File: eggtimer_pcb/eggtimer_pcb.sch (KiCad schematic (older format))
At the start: 84 parts, among them J1 Conn_01x03, Q1 CPH3350-TL-W, Q10 2N7002P,215, Q2 CPH3350-TL-W, Q3 CPH3350-TL-W, Q4 CPH3350-TL-W, Q5 CPH3350-TL-W, Q6 CPH3350-TL-W, Q7 CPH3350-TL-W, Q8 CPH3350-TL-W, Q9 2N7002P,215, SW1 Rotary_Encoder_Switch, SW2 SW_Push, U1 BD70522GUL-E2, U2 STM32G051GxU, Y1 32.xxxk

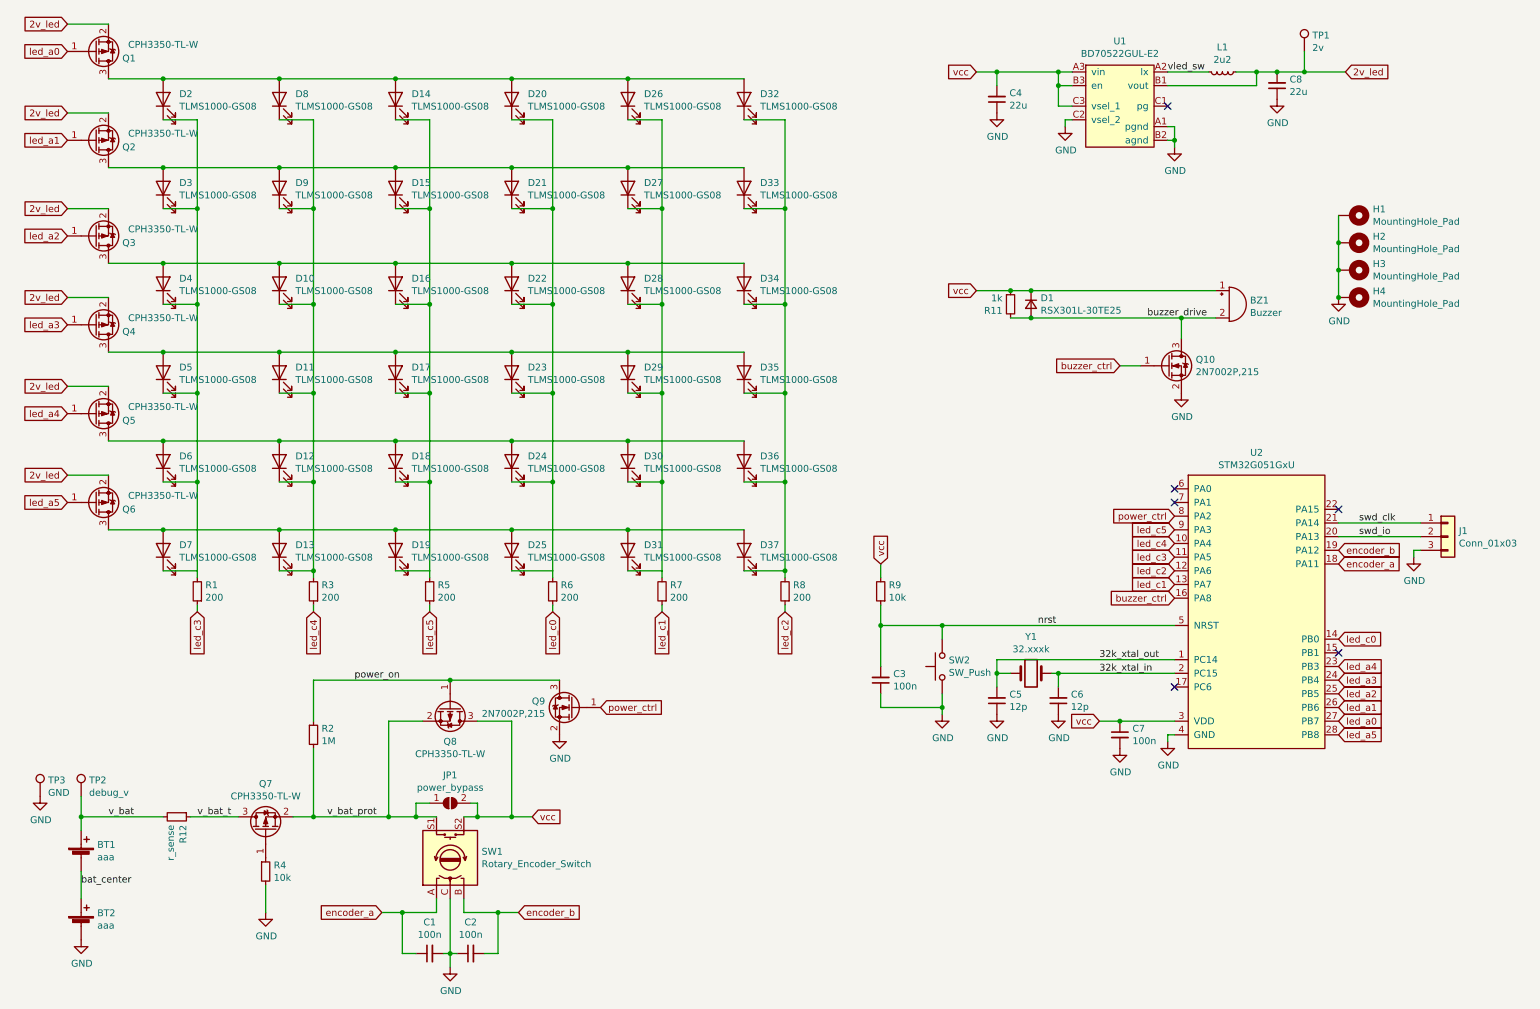
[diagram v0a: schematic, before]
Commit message: MORE LEDS
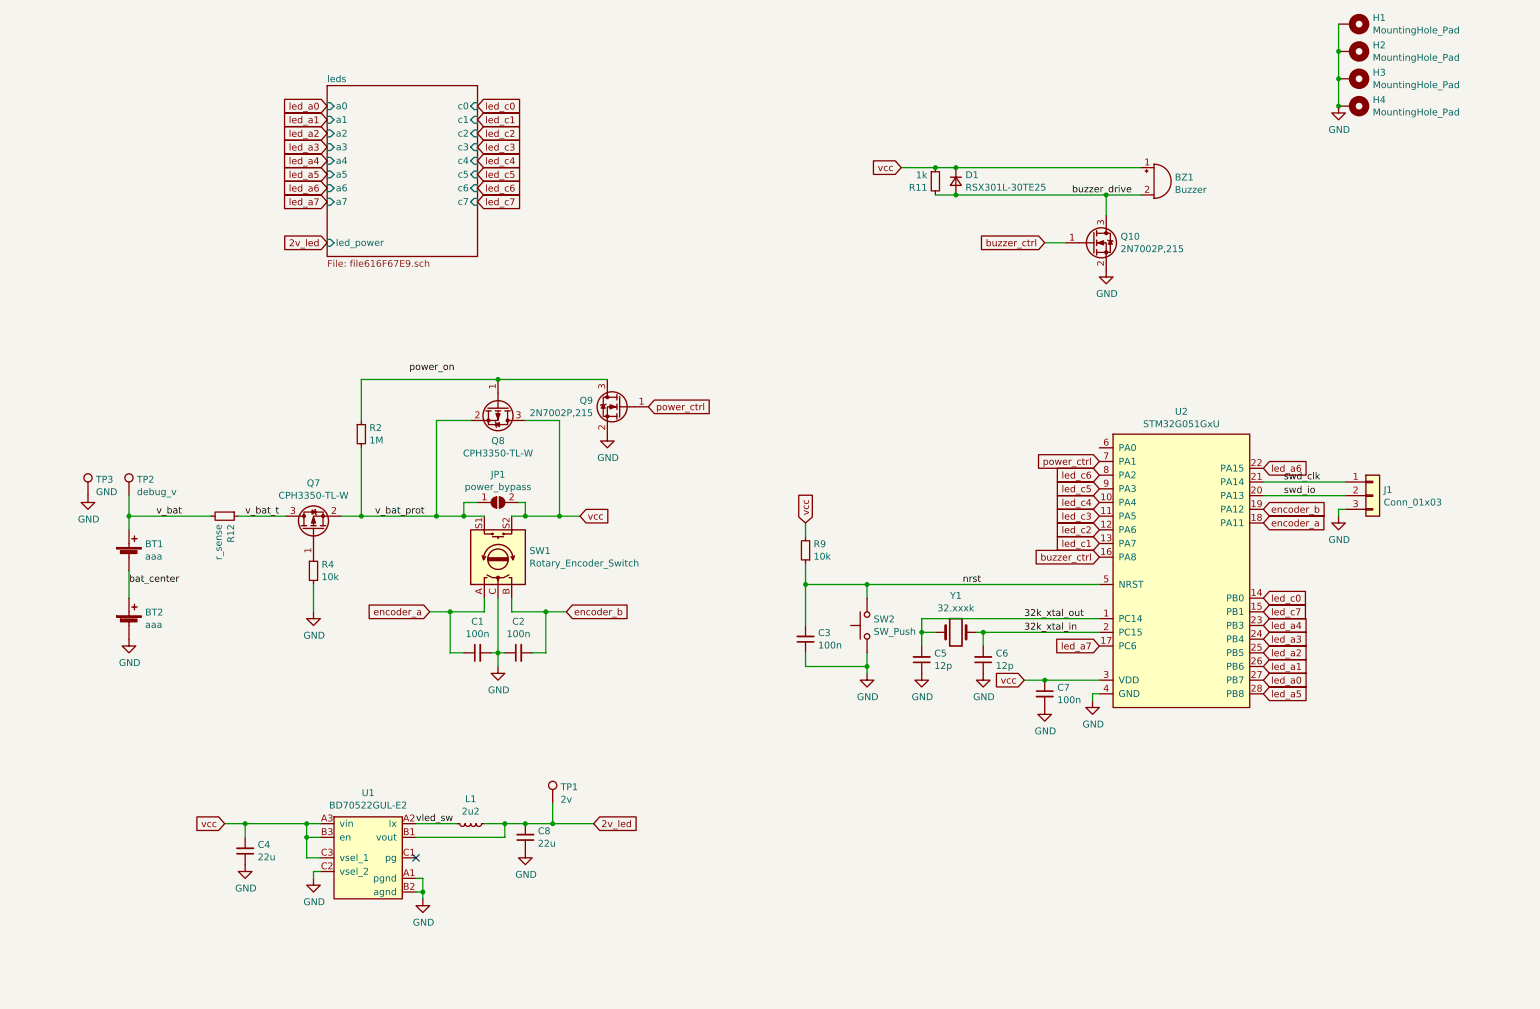
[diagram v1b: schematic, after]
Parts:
- removed D10, D11, D12, D13, D14, D15, D16, D17, D18, D19, D2, D20, D21, D22, D23, D24, D25, D26, D27, D28, D29, D3, D30, D31, D32, D33, D34, D35, D36, D37, D4, D5, D6, D7, D8, D9: TLMS1000-GS08, LED_SMD:LED_0603_1608Metric_Pad1.05x0.95mm_HandSolder, symbol Device:LED
- removed Q1, Q2, Q3, Q4, Q5, Q6: CPH3350-TL-W, Package_TO_SOT_SMD:SOT-23_Handsoldering, symbol Device:Q_PMOS_GSD
- removed R1, R3, R5, R6, R7, R8: 200, Resistor_SMD:R_0603_1608Metric_Pad0.98x0.95mm_HandSolder, symbol Device:R_Small
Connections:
- net power_ctrl: now also U2.7 (PA1); no longer U2.8 (PA2)
- net power_on: no longer Q8.1 (G), Q9.3 (D), R2.1
- net led_c7: now reaches U2.15 (PB1)
- net led_a7: now reaches U2.17 (PC6)
- net led_a6: now reaches U2.22 (PA15)
- new net: Q8.1 (G), Q9.3 (D), R2.1
- new net led_c6: U2.8 (PA2)
- no-connect marks 6 -> 1
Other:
- moved on the sheet: BT1, BT2, BZ1, C1, C2, C3, C4, C5, C6, C7, C8, D1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
